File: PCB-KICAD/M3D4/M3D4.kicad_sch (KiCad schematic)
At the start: 29 parts, among them J1 USB_B, P2 STDCONN, U1 CM108AH, U4 93CxxA, U5 AMS1117-5.0, U6 AMS1117-3.3, Y1 12MHz

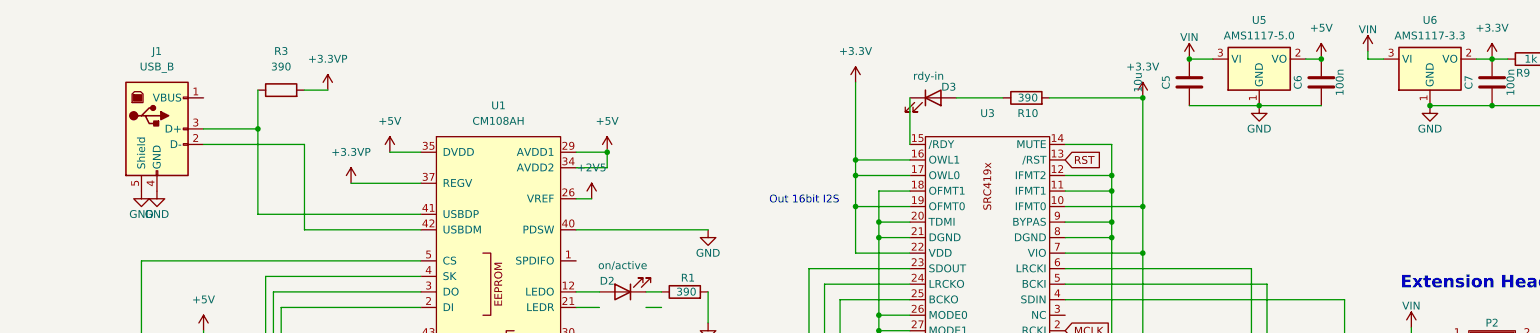
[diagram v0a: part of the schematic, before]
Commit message: First test board.
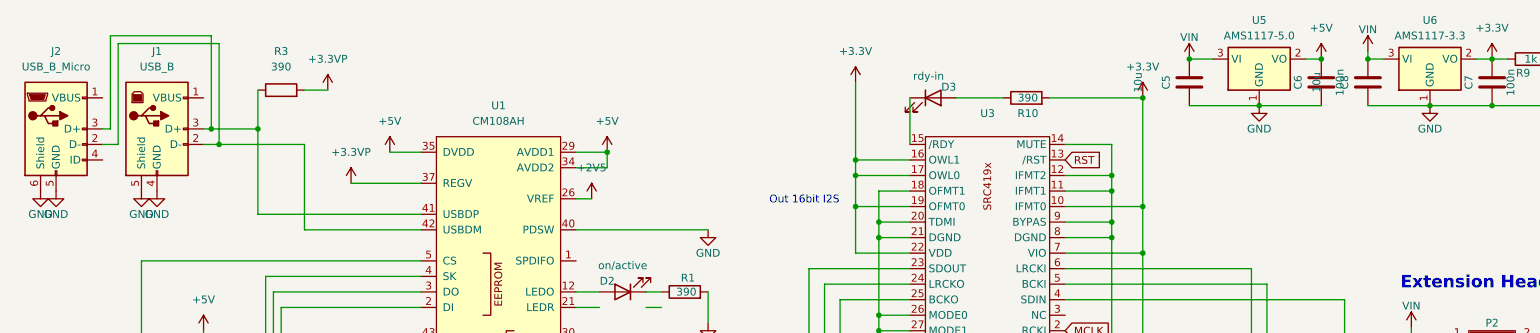
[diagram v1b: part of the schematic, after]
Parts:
- added C8: 10u, Capacitor_SMD:C_1206_3216Metric_Pad1.33x1.80mm_HandSolder, symbol Device:C
- added J2: USB_B_Micro, Connector_USB:USB_Micro-B_Amphenol_10103594-0001LF_Horizontal, symbol Connector:USB_B_Micro
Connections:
- net GND: now also C8.2, J2.5 (GND), J2.6 (Shield)
- net VIN: now also C8.1
- net at J1.2 (D-), U1.42 (USBDM): now also J2.2 (D-)
- net at J1.3 (D+), R3.1, U1.41 (USBDP): now also J2.3 (D+)
